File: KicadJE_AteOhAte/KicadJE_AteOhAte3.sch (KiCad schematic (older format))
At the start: 65 parts, among them J301 Out 1, J303 Out 2, J305 Out 1 Final, J306 Out 2 Final, U301 TL072, U302 TL072

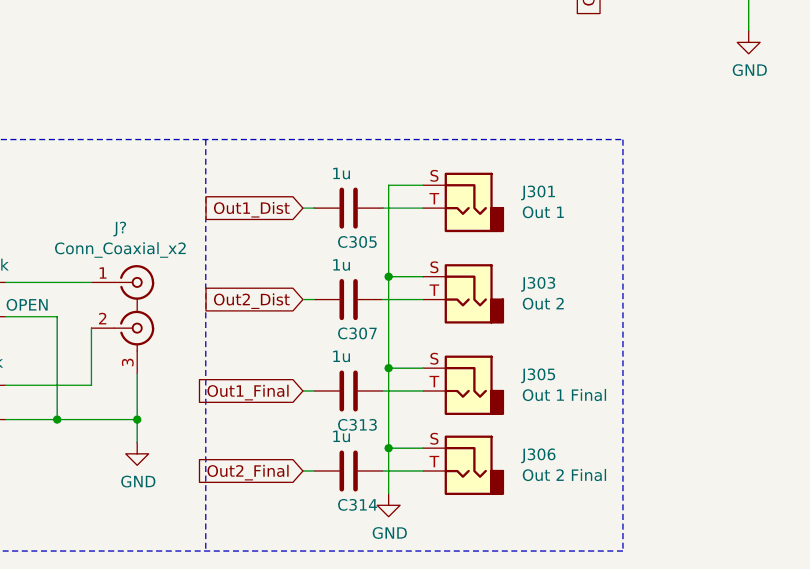
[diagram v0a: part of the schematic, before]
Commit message: RCA on RIAA
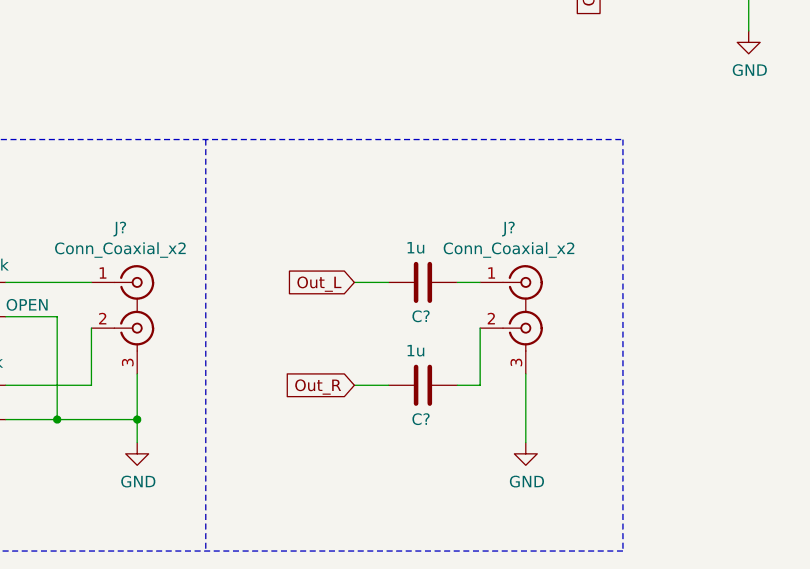
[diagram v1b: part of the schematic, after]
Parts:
- removed C305, C307, C313, C314: 1u, Capacitor_SMD:C_0805_2012Metric_Pad1.15x1.40mm_HandSolder, symbol Device:C
- removed J301: Out 1, AJ-Dropbox-Kicad:PJ301SM, symbol Connector:AudioJack2
- removed J303: Out 2, AJ-Dropbox-Kicad:PJ301SM, symbol Connector:AudioJack2
- removed J305: Out 1 Final, AJ-Dropbox-Kicad:PJ301SM, symbol Connector:AudioJack2
- removed J306: Out 2 Final, AJ-Dropbox-Kicad:PJ301SM, symbol Connector:AudioJack2
- added C? (x2): 1u, Capacitor_SMD:C_0805_2012Metric_Pad1.15x1.40mm_HandSolder, symbol Device:C
- added J?: Conn_Coaxial_x2, symbol Connector:Conn_Coaxial_x2
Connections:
- net labels added: Out_L, Out_R
- wire segments 155 -> 145
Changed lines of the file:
@@
 	2125 6575 2525 6575
-$Comp
-L Connector:AudioJack2 J?
-U 1 1 5D7994F9
-P 6250 6225
-AR Path="/5CF11B19/5D7994F9" Ref="J?"  Part="1"
-AR Path="/5D4DB615/5D7994F9" Ref="J301"  Part="1"
-F 0 "J301" H 6017 6296 50  0000 R CNN
-F 1 "Out 1" H 6017 6205 50  0000 R CNN
-F 2 "AJ-Dropbox-Kicad:PJ301SM" H 6250 6225 50  0001 C CNN
-F 3 "~" H 6250 6225 50  0001 C CNN
-	1    6250 6225
-	-1   0    0    -1
-$EndComp
-$Comp
-L Connector:AudioJack2 J?
-U 1 1 5D7994FF
-P 6250 6625
-AR Path="/5CF11B19/5D7994FF" Ref="J?"  Part="1"
-AR Path="/5D4DB615/5D7994FF" Ref="J303"  Part="1"
-F 0 "J303" H 6017 6696 50  0000 R CNN
-F 1 "Out 2" H 6017 6605 50  0000 R CNN
-F 2 "AJ-Dropbox-Kicad:PJ301SM" H 6250 6625 50  0001 C CNN
-F 3 "~" H 6250 6625 50  0001 C CNN
-	1    6250 6625
-	-1   0    0    -1
-$EndComp
-Wire Wire Line
-	6050 6125 5900 6125
-Wire Wire Line
-	6050 6525 5900 6525
 $Comp
 L Device:R R?
@@
 	0    -1   -1   0
 $EndComp
-Wire Wire Line
-	5900 6125 5900 6525
 Connection ~ 3875 6550
 Wire Wire Line
@@
 $Comp
 L power:GND #PWR?
-U 1 1 5D79953C
-P 5900 7475
-AR Path="/5CF11B19/5D79953C" Ref="#PWR?"  Part="1"
-AR Path="/5D4DB615/5D79953C" Ref="#PWR0314"  Part="1"
-F 0 "#PWR0314" H 5900 7225 50  0001 C CNN
-F 1 "GND" H 5905 7302 50  0000 C CNN
-F 2 "" H 5900 7475 50  0001 C CNN
-F 3 "" H 5900 7475 50  0001 C CNN
-	1    5900 7475
-	1    0    0    -1
-$EndComp
-Text GLabel 5525 6625 0    50   Input ~ 0
-Out2_Dist
-Text GLabel 5525 6225 0    50   Input ~ 0
-Out1_Dist
-$Comp
-L power:GND #PWR?
 U 1 1 5D799544
 P 4800 7250
@@
 	0    1    1    0
 $EndComp
-$Comp
-L Connector:AudioJack2 J?
-U 1 1 5D79956C
-P 6250 7375
-AR Path="/5CF11B19/5D79956C" Ref="J?"  Part="1"
-AR Path="/5D4DB615/5D79956C" Ref="J306"  Part="1"
-F 0 "J306" H 6017 7446 50  0000 R CNN
-F 1 "Out 2 Final" H 6017 7355 50  0000 R CNN
-F 2 "AJ-Dropbox-Kicad:PJ301SM" H 6250 7375 50  0001 C CNN
-F 3 "~" H 6250 7375 50  0001 C CNN
-	1    6250 7375
-	-1   0    0    -1
-$EndComp
-Wire Wire Line
-	6050 7275 5900 7275
-Wire Wire Line
-	5900 7475 5900 7275
-Wire Wire Line
-	5900 6525 5900 6925
-Text GLabel 5525 7375 0    50   Input ~ 0
-Out2_Final
-Connection ~ 5900 6525
 Wire Wire Line
 	1850 6575 2125 6575
@@
 Wire Wire Line
 	8125 4550 8275 4550
-$Comp
-L Connector:AudioJack2 J?
-U 1 1 5D84994A
-P 6250 7025
-AR Path="/5CF11B19/5D84994A" Ref="J?"  Part="1"
-AR Path="/5D4DB615/5D84994A" Ref="J305"  Part="1"
-F 0 "J305" H 6017 7096 50  0000 R CNN
-F 1 "Out 1 Final" H 6017 7005 50  0000 R CNN
-F 2 "AJ-Dropbox-Kicad:PJ301SM" H 6250 7025 50  0001 C CNN
-F 3 "~" H 6250 7025 50  0001 C CNN
-	1    6250 7025
-	-1   0    0    -1
-$EndComp
-Text GLabel 5525 7025 0    50   Input ~ 0
-Out1_Final
-Wire Wire Line
-	6050 6925 5900 6925
-Wire Wire Line
-	5900 7275 5900 6925
-Connection ~ 5900 7275
-Connection ~ 5900 6925
 Text GLabel 8975 4550 2    50   Input ~ 0
 Out2_Final
@@
 Wire Wire Line
 	6775 4875 6775 4950
-$Comp
-L Device:C C?
-U 1 1 5D8781E6
-P 5725 6225
-AR Path="/5CF11B19/5D8781E6" Ref="C?"  Part="1"
-AR Path="/5D4DB615/5D8781E6" Ref="C305"  Part="1"
-F 0 "C305" V 5875 6175 50  0000 L CNN
-F 1 "1u" V 5575 6150 50  0000 L CNN
-F 2 "Capacitor_SMD:C_0805_2012Metric_Pad1.15x1.40mm_HandSolder" H 5763 6075 50  0001 C CNN
-F 3 "~" H 5725 6225 50  0001 C CNN
-	1    5725 6225
-	0    1    1    0
-$EndComp
-Wire Wire Line
-	5525 6225 5575 6225
-Wire Wire Line
-	5525 6625 5575 6625
-Wire Wire Line
-	5525 7025 5575 7025
-Wire Wire Line
-	5525 7375 5575 7375
-Wire Wire Line
-	5875 6225 6050 6225
-$Comp
-L Device:C C?
-U 1 1 5D88B3A1
-P 5725 6625
-AR Path="/5CF11B19/5D88B3A1" Ref="C?"  Part="1"
-AR Path="/5D4DB615/5D88B3A1" Ref="C307"  Part="1"
-F 0 "C307" V 5875 6575 50  0000 L CNN
-F 1 "1u" V 5575 6550 50  0000 L CNN
-F 2 "Capacitor_SMD:C_0805_2012Metric_Pad1.15x1.40mm_HandSolder" H 5763 6475 50  0001 C CNN
-F 3 "~" H 5725 6625 50  0001 C CNN
-	1    5725 6625
-	0    1    1    0
-$EndComp
-Wire Wire Line
-	5875 6625 6050 6625
-$Comp
-L Device:C C?
-U 1 1 5D88B72B
-P 5725 7025
-AR Path="/5CF11B19/5D88B72B" Ref="C?"  Part="1"
-AR Path="/5D4DB615/5D88B72B" Ref="C313"  Part="1"
-F 0 "C313" V 5875 6975 50  0000 L CNN
-F 1 "1u" V 5575 6950 50  0000 L CNN
-F 2 "Capacitor_SMD:C_0805_2012Metric_Pad1.15x1.40mm_HandSolder" H 5763 6875 50  0001 C CNN
-F 3 "~" H 5725 7025 50  0001 C CNN
-	1    5725 7025
-	0    1    1    0
-$EndComp
-Wire Wire Line
-	5875 7025 6050 7025
-$Comp
-L Device:C C?
-U 1 1 5D88BB07
-P 5725 7375
-AR Path="/5CF11B19/5D88BB07" Ref="C?"  Part="1"
-AR Path="/5D4DB615/5D88BB07" Ref="C314"  Part="1"
-F 0 "C314" V 5875 7325 50  0000 L CNN
-F 1 "1u" V 5575 7300 50  0000 L CNN
-F 2 "Capacitor_SMD:C_0805_2012Metric_Pad1.15x1.40mm_HandSolder" H 5763 7225 50  0001 C CNN
-F 3 "~" H 5725 7375 50  0001 C CNN
-	1    5725 7375
-	0    1    1    0
-$EndComp
-Wire Wire Line
-	5875 7375 6050 7375
 $Comp
 L power:GND #PWR?
@@
 Text GLabel 2825 3525 0    50   Input ~ 0
 In_R
+$Comp
+L power:GND #PWR?
+U 1 1 5DC3A5B0
+P 6500 7250
+AR Path="/5CF11B19/5DC3A5B0" Ref="#PWR?"  Part="1"
+AR Path="/5D4DB615/5DC3A5B0" Ref="#PWR?"  Part="1"
+F 0 "#PWR?" H 6500 7000 50  0001 C CNN
+F 1 "GND" H 6505 7077 50  0000 C CNN
+F 2 "" H 6500 7250 50  0001 C CNN
+F 3 "" H 6500 7250 50  0001 C CNN
+	1    6500 7250
+	1    0    0    -1
+$EndComp
+Text GLabel 5750 6550 0    50   Input ~ 0
+Out_L
+Text GLabel 5750 7000 0    50   Input ~ 0
+Out_R
+Wire Wire Line
+	5750 7000 5900 7000
+Wire Wire Line
+	5750 6550 5900 6550
+$Comp
+L Device:C C?
+U 1 1 5DC3A5BE
+P 6050 6550
+AR Path="/5CF11B19/5DC3A5BE" Ref="C?"  Part="1"
+AR Path="/5D4DB615/5DC3A5BE" Ref="C?"  Part="1"
+F 0 "C?" V 6200 6500 50  0000 L CNN
+F 1 "1u" V 5900 6475 50  0000 L CNN
+F 2 "Capacitor_SMD:C_0805_2012Metric_Pad1.15x1.40mm_HandSolder" H 6088 6400 50  0001 C CNN
+F 3 "~" H 6050 6550 50  0001 C CNN
+	1    6050 6550
+	0    1    1    0
+$EndComp
+$Comp
+L Device:C C?
+U 1 1 5DC3A5C8
+P 6050 7000
+AR Path="/5CF11B19/5DC3A5C8" Ref="C?"  Part="1"
+AR Path="/5D4DB615/5DC3A5C8" Ref="C?"  Part="1"
+F 0 "C?" V 6200 6950 50  0000 L CNN
+F 1 "1u" V 5900 6925 50  0000 L CNN
+F 2 "Capacitor_SMD:C_0805_2012Metric_Pad1.15x1.40mm_HandSolder" H 6088 6850 50  0001 C CNN
+F 3 "~" H 6050 7000 50  0001 C CNN
+	1    6050 7000
+	0    1    1    0
+$EndComp
+$Comp
+L Connector:Conn_Coaxial_x2 J?
+U 1 1 5DC3A5D2
+P 6500 6650
+F 0 "J?" H 6428 6988 50  0000 C CNN
+F 1 "Conn_Coaxial_x2" H 6428 6897 50  0000 C CNN
+F 2 "" H 6500 6550 50  0001 C CNN
+F 3 " ~" H 6500 6550 50  0001 C CNN
+	1    6500 6650
+	1    0    0    -1
+$EndComp
+Wire Wire Line
+	6300 7000 6300 6750
+Wire Wire Line
+	6500 6950 6500 7250
+Wire Wire Line
+	6200 6550 6300 6550
+Wire Wire Line
+	6300 7000 6200 7000
 $EndSCHEMATC

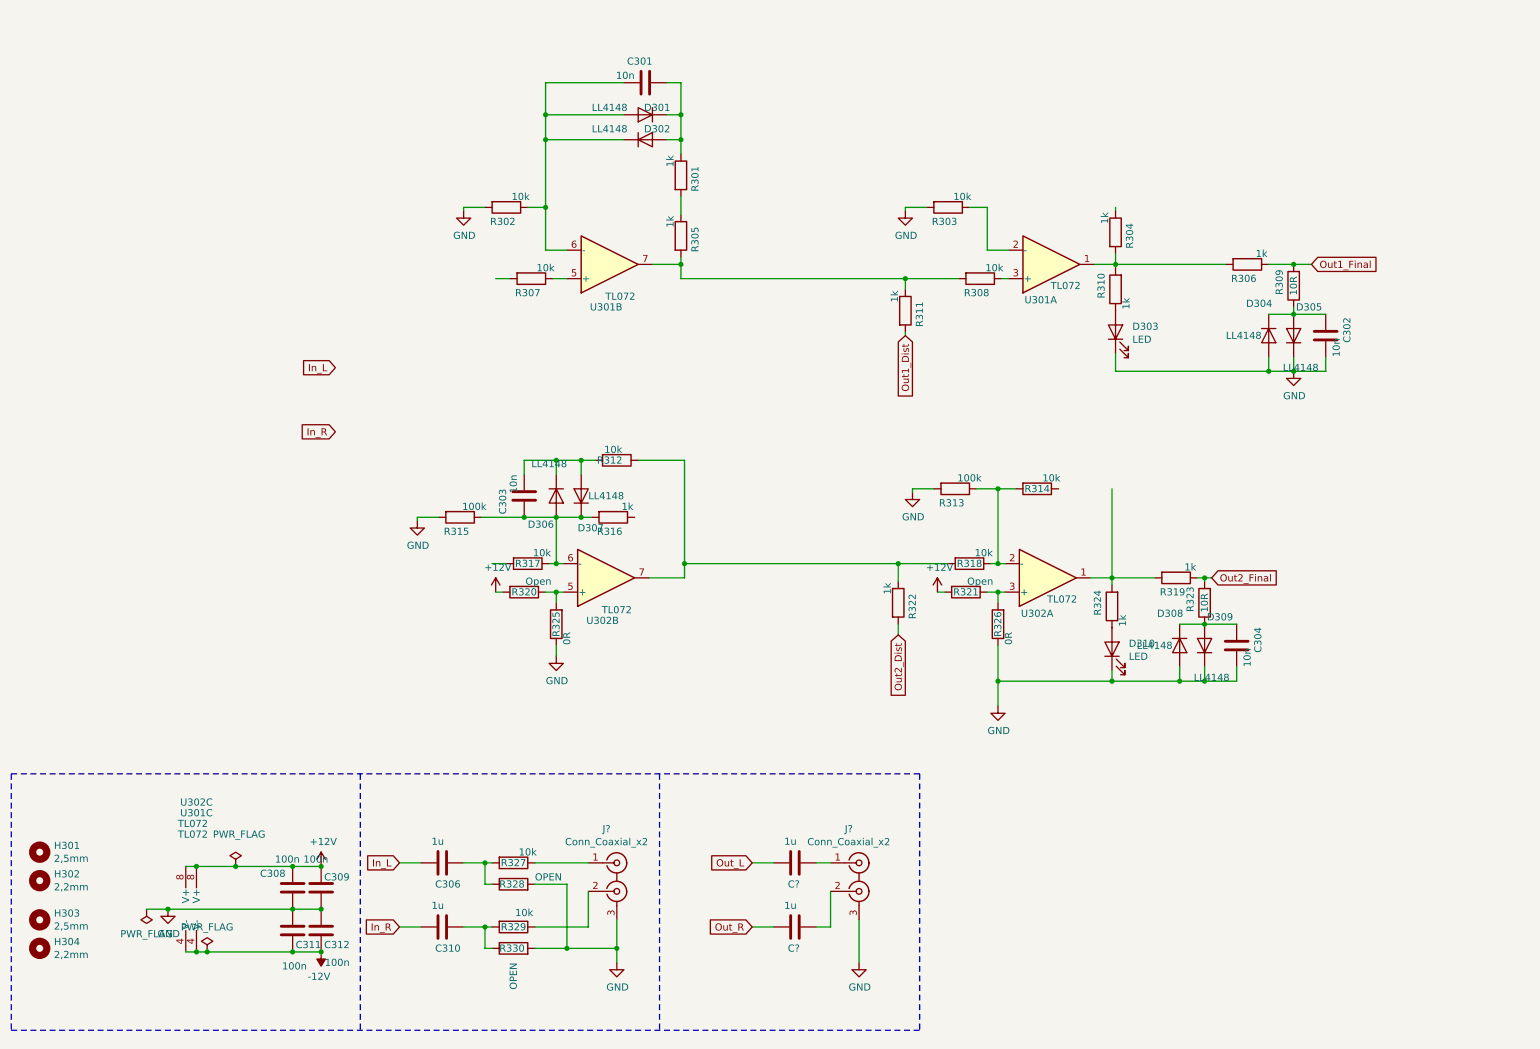
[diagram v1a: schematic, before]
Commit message: RIAA Basic Circuit
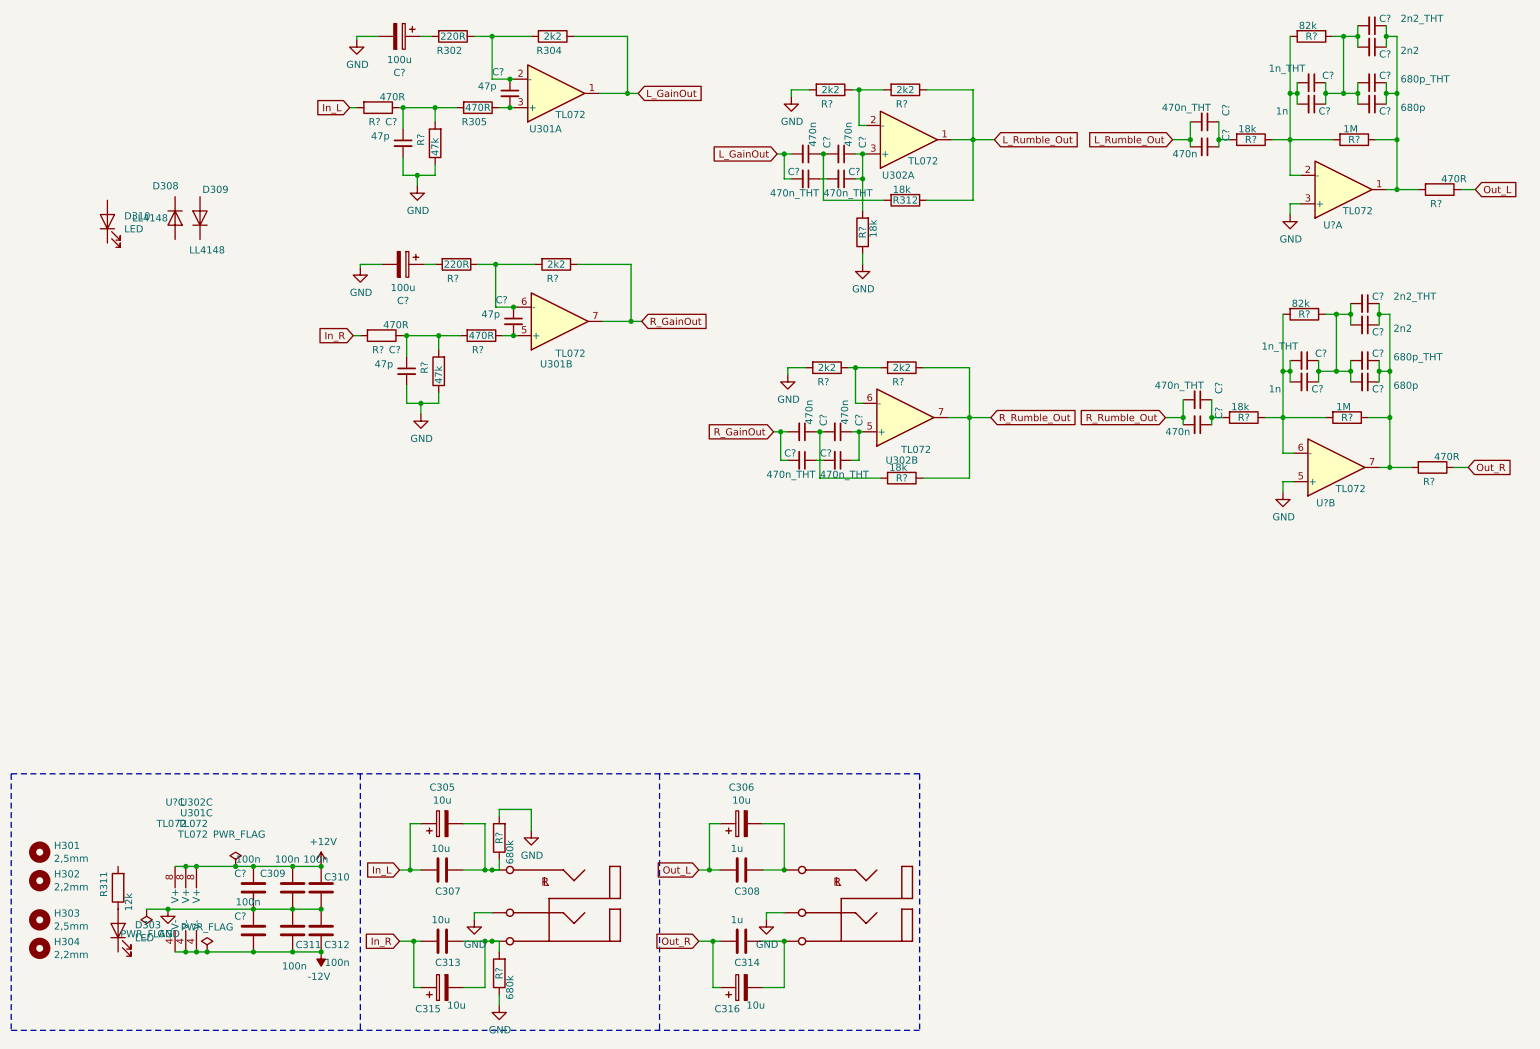
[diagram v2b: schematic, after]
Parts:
- removed C301, C302, C303, C304: 10n, Capacitor_SMD:C_0805_2012Metric_Pad1.15x1.40mm_HandSolder, symbol Device:C
- removed D301, D302, D304, D305, D306, D307: LL4148, Diode_SMD:D_MiniMELF, symbol Diode:LL4148
- removed J? (x2): Conn_Coaxial_x2, symbol Connector:Conn_Coaxial_x2
- removed R301, R304, R306, R311, R316, R319, R322, R324: 1k, Resistor_SMD:R_0805_2012Metric_Pad1.15x1.40mm_HandSolder, symbol Device:R
- removed R303, R308, R314, R317, R318, R327, R329: 10k, Resistor_SMD:R_0805_2012Metric_Pad1.15x1.40mm_HandSolder, symbol Device:R
- removed R309, R323: 10R, Resistor_SMD:R_0805_2012Metric_Pad1.15x1.40mm_HandSolder, symbol Device:R
- removed R313, R315: 100k, Resistor_SMD:R_0805_2012Metric_Pad1.15x1.40mm_HandSolder, symbol Device:R
- removed R320, R321: Open, Resistor_SMD:R_0805_2012Metric_Pad1.15x1.40mm_HandSolder, symbol Device:R
- removed R325, R326: 0R, Resistor_SMD:R_0805_2012Metric_Pad1.15x1.40mm_HandSolder, symbol Device:R
- removed R328, R330: OPEN, Resistor_SMD:R_0805_2012Metric_Pad1.15x1.40mm_HandSolder, symbol Device:R
- added C305, C306, C315, C316: 10u, Capacitor_THT:CP_Radial_D6.3mm_P2.50mm, symbol Device:CP
- added C? (x4): 47p, symbol Device:C_Small
- added C? (x2): 100u, Capacitor_THT:CP_Radial_D6.3mm_P2.50mm, symbol Device:CP
- added C? (x4): 470n, symbol Device:C_Small
- added C? (x6): 470n_THT, Capacitor_THT:C_Rect_L7.2mm_W5.5mm_P5.00mm_FKS2_FKP2_MKS2_MKP2, symbol Device:C_Small
- added C? (x2): 470n, Capacitor_SMD:C_1206_3216Metric_Pad1.42x1.75mm_HandSolder, symbol Device:C_Small
- added C? (x2): 1n_THT, Capacitor_THT:C_Rect_L7.2mm_W5.5mm_P5.00mm_FKS2_FKP2_MKS2_MKP2, symbol Device:C_Small
- added C? (x2): 1n, Capacitor_SMD:C_1206_3216Metric_Pad1.42x1.75mm_HandSolder, symbol Device:C_Small
- added C? (x2): 680p_THT, Capacitor_THT:C_Rect_L7.2mm_W5.5mm_P5.00mm_FKS2_FKP2_MKS2_MKP2, symbol Device:C_Small
- added C? (x2): 680p, Capacitor_SMD:C_1206_3216Metric_Pad1.42x1.75mm_HandSolder, symbol Device:C_Small
- added C? (x2): 2n2_THT, Capacitor_THT:C_Rect_L7.2mm_W5.5mm_P5.00mm_FKS2_FKP2_MKS2_MKP2, symbol Device:C_Small
- added C? (x2): 2n2, Capacitor_SMD:C_1206_3216Metric_Pad1.42x1.75mm_HandSolder, symbol Device:C_Small
- added C? (x2): 100n, Capacitor_SMD:C_0805_2012Metric_Pad1.15x1.40mm_HandSolder, symbol Device:C
- added J301: PJRAS2X2S01AUX, PJRAS2X2S01AUX, symbol PJRAS2X2S01AUX:PJRAS2X2S01AUX
- added R? (x2): 680k, Resistor_SMD:R_0805_2012Metric_Pad1.15x1.40mm_HandSolder, symbol Device:R
- added R? (x5): 470R, Resistor_SMD:R_0805_2012Metric_Pad1.15x1.40mm_HandSolder, symbol Device:R
- added R? (x2): 47k, Resistor_SMD:R_0805_2012Metric_Pad1.15x1.40mm_HandSolder, symbol Device:R
- added R? (x5): 2k2, Resistor_SMD:R_0805_2012Metric_Pad1.15x1.40mm_HandSolder, symbol Device:R
- added R?: 220R, Resistor_SMD:R_0805_2012Metric_Pad1.15x1.40mm_HandSolder, symbol Device:R
- added R? (x4): 18k, Resistor_SMD:R_0805_2012Metric_Pad1.15x1.40mm_HandSolder, symbol Device:R
- added R? (x2): 1M, Resistor_SMD:R_0805_2012Metric_Pad1.15x1.40mm_HandSolder, symbol Device:R
- added R? (x2): 82k, Resistor_SMD:R_0805_2012Metric_Pad1.15x1.40mm_HandSolder, symbol Device:R
- added U? (x3): TL072, AJ-Dropbox-Kicad:AJ_SO-8_5.3x6.2mm_P1.27mm, symbol Amplifier_Operational:TL072
- C307: renamed from C306; value 1u -> 10u
- C313: renamed from C310; value 1u -> 10u
- R302: value 10k -> 220R
- R304: renamed from R305; value 1k -> 2k2
- R305: renamed from R307; value 10k -> 470R
- R311: renamed from R310; value 1k -> 12k
- R312: value 10k -> 18k
- gave numbers to parts that had none: 2
- renumbered C308 to C309, C309 to C310
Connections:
- net labels added: L_GainOut, L_Rumble_Out, R_GainOut, R_Rumble_Out
- net labels removed: Out1_Dist, Out1_Final, Out2_Dist, Out2_Final
- wire segments 145 -> 242
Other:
- moved on the sheet: C307, C308, C313, C314, D303, D308, D309, D310, R302, R304, R305, R311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
